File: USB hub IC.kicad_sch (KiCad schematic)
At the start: 4 parts, among them U1 FE1.1s, U2 FE1.1s

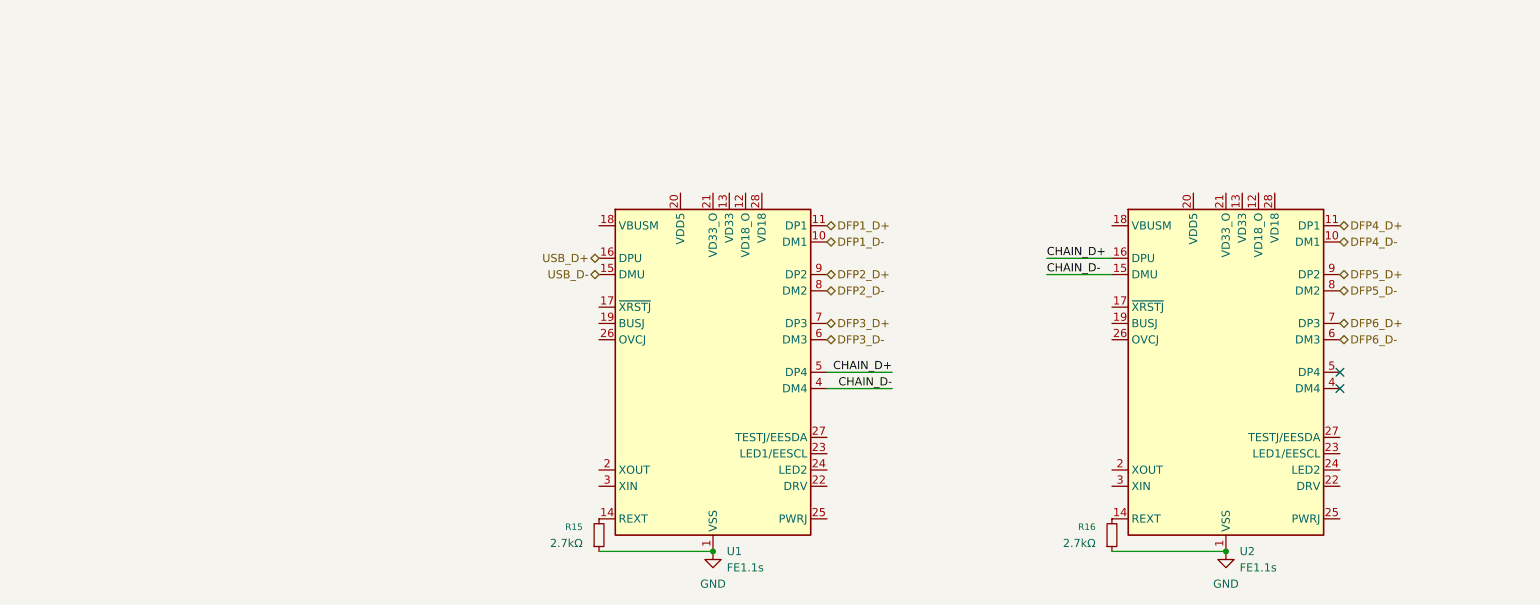
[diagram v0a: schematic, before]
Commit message: more work on USB hubs
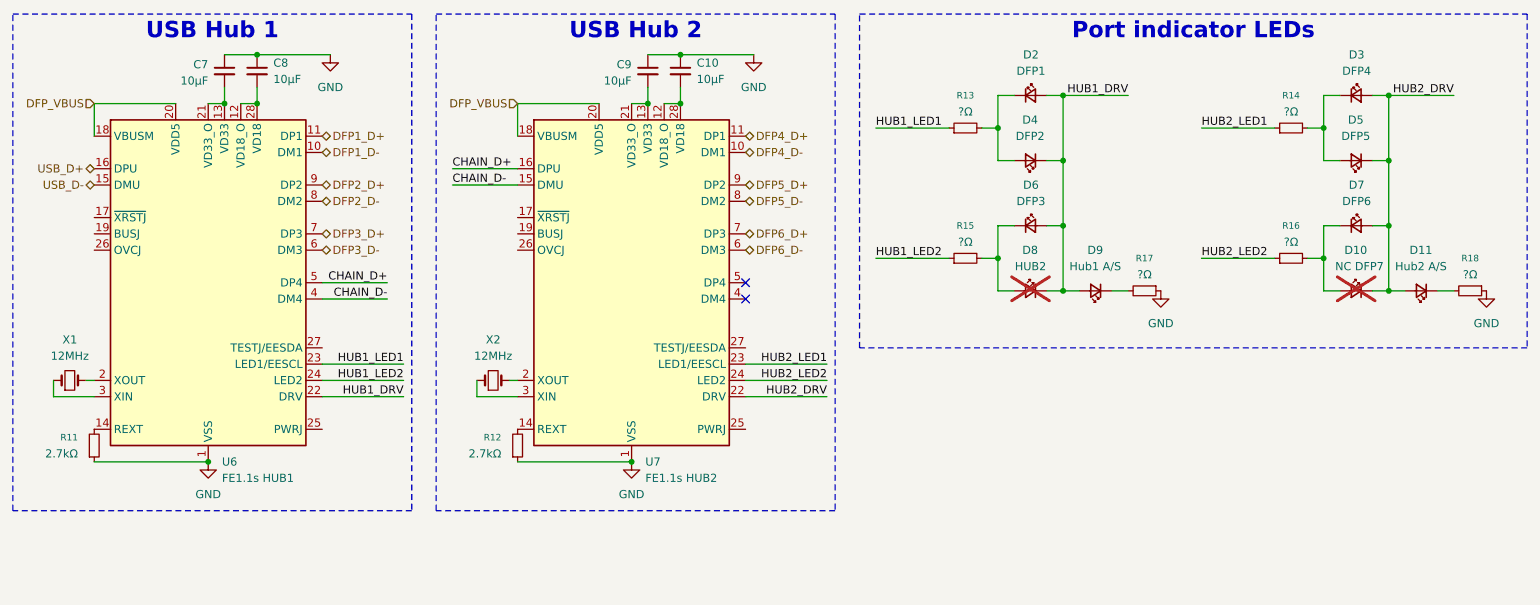
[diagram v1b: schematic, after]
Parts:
- added C10, C7, C8, C9: 10μF, symbol Device:C_Small
- added D10: NC DFP7, symbol Device:LED_Small
- added D11: Hub2 A/S, symbol Device:LED_Small
- added D2: DFP1, symbol Device:LED_Small
- added D3: DFP4, symbol Device:LED_Small
- added D4: DFP2, symbol Device:LED_Small
- added D5: DFP5, symbol Device:LED_Small
- added D6: DFP3, symbol Device:LED_Small
- added D7: DFP6, symbol Device:LED_Small
- added D8: HUB2, symbol Device:LED_Small
- added D9: Hub1 A/S, symbol Device:LED_Small
- added R13, R14, R15, R16, R17, R18: ?Ω, symbol Device:R_Small
- added X1, X2: 12MHz, symbol Device:Crystal_Small
- U6: renamed from U1; value FE1.1s -> FE1.1s HUB1
- U7: renamed from U2; value FE1.1s -> FE1.1s HUB2
- renumbered R15 to R11, R16 to R12
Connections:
- net GND: now also C10.1, C7.1, C8.1, C9.1, R17.1, R18.1
- net at U7.12 (VD18_O): now also U7.28 (VD18), C10.2
- net at U7.13 (VD33): now also U7.21 (VD33_O), C9.2
- net DFP_VBUS: now reaches U7.18 (VBUSM)
- net DFP_VBUS: now also U6.18 (VBUSM), U6.20 (VDD5), U7.20 (VDD5)
- net at U7.2 (XOUT): now also X2.2
- net HUB2_DRV: now reaches U7.22 (DRV)
- net HUB2_DRV: now also D10.1 (K), D11.2 (A), D3.2 (A), D5.1 (K), D7.2 (A)
- net HUB2_LED1: now reaches U7.23 (LED1/EESCL)
- net HUB2_LED1: now also R14.1
- net HUB2_LED2: now reaches U7.24 (LED2)
- net HUB2_LED2: now also R16.1
- net at U7.3 (XIN): now also X2.1
- net at U6.12 (VD18_O): now also U6.28 (VD18), C8.2
- net at U6.13 (VD33): now also U6.21 (VD33_O), C7.2
- net at U6.2 (XOUT): now also X1.2
- net HUB1_DRV: now reaches U6.22 (DRV)
- net HUB1_DRV: now also D2.2 (A), D4.1 (K), D6.2 (A), D8.1 (K), D9.2 (A)
- net HUB1_LED1: now reaches U6.23 (LED1/EESCL)
- net HUB1_LED1: now also R13.1
- net HUB1_LED2: now reaches U6.24 (LED2)
- net HUB1_LED2: now also R15.1
- net at U6.3 (XIN): now also X1.1
- new net: D6.1 (K), D8.2 (A), R15.2
- new net: D2.1 (K), D4.2 (A), R13.2
- new net: D10.2 (A), D7.1 (K), R16.2
- new net: D3.1 (K), D5.2 (A), R14.2
- new net: D11.1 (K), R18.2
- new net: D9.1 (K), R17.2
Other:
- moved on the sheet: R11, R12, U6, U7
